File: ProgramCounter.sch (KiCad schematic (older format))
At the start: 8 parts, among them U13 74LS245, U14 74LS245, U15 74LS161, U16 74LS161, U17 74LS161, U18 74LS161

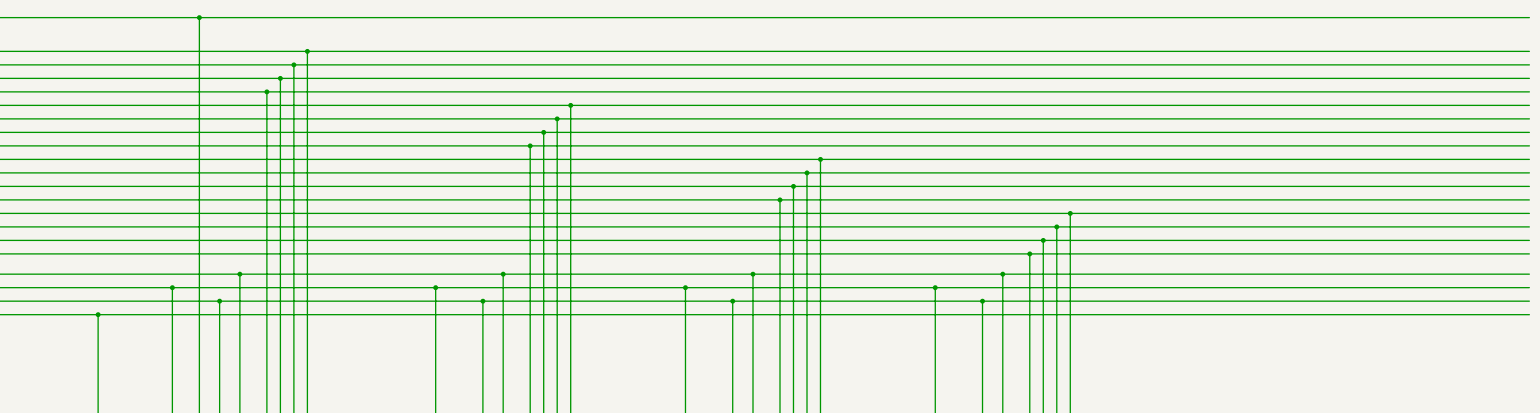
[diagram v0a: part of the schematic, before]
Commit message: clean up
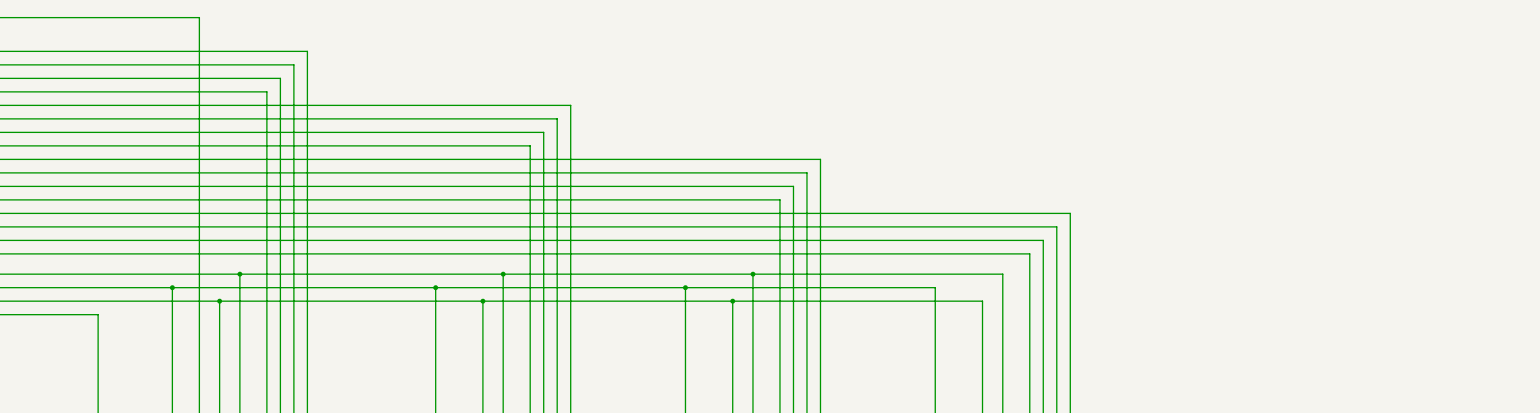
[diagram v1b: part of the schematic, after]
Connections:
- wire segments 243 -> 222
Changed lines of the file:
@@
 Wire Wire Line
 	9400 2750 11250 2750
-Connection ~ 11250 2750
-Wire Wire Line
-	11250 2750 15650 2750
 Wire Wire Line
 	1150 2750 5600 2750
@@
 Wire Wire Line
 	11750 3950 11750 2650
-Connection ~ 11750 2650
-Wire Wire Line
-	11750 2650 15650 2650
 Wire Wire Line
 	5800 3950 5800 750
-Connection ~ 5800 750
-Wire Wire Line
-	5800 750  15650 750
 Text HLabel 1150 2850 0    50   Input ~ 0
 CE
@@
 Wire Wire Line
 	11650 3900 11650 3950
-Connection ~ 11600 2850
-Wire Wire Line
-	11600 2850 15650 2850
 Wire Wire Line
 	11600 3900 11550 3900
@@
 Wire Wire Line
 	4450 5150 4450 4950
-Connection ~ 5050 2950
-Wire Wire Line
-	5050 2950 15650 2950
 Wire Wire Line
 	6600 3950 6600 1000
-Connection ~ 6600 1000
-Wire Wire Line
-	6600 1000 15650 1000
 Wire Wire Line
 	6500 3950 6500 1100
-Connection ~ 6500 1100
-Wire Wire Line
-	6500 1100 15650 1100
 Wire Wire Line
 	6400 3950 6400 1200
-Connection ~ 6400 1200
-Wire Wire Line
-	6400 1200 15650 1200
 Wire Wire Line
 	6300 3950 6300 1300
-Connection ~ 6300 1300
-Wire Wire Line
-	6300 1300 15650 1300
-Connection ~ 8550 1400
 Wire Wire Line
 	8450 1500 8450 3950
-Connection ~ 8450 1500
-Wire Wire Line
-	8450 1500 15650 1500
 Wire Wire Line
 	8350 1600 8350 3950
-Connection ~ 8350 1600
-Wire Wire Line
-	8350 1600 15650 1600
 Connection ~ 8550 3950
 Wire Wire Line
@@
 Wire Wire Line
 	2550 1700 8250 1700
-Connection ~ 8250 1700
-Wire Wire Line
-	8250 1700 15650 1700
-Wire Wire Line
-	8550 1400 15650 1400
 Wire Wire Line
 	8250 3950 8250 1700
@@
 Wire Wire Line
 	10400 3950 10400 1800
-Connection ~ 10400 1800
-Wire Wire Line
-	10400 1800 15650 1800
 Wire Wire Line
 	10300 3950 10300 1900
-Connection ~ 10300 1900
-Wire Wire Line
-	10300 1900 15650 1900
 Wire Wire Line
 	10200 3950 10200 2000
-Connection ~ 10200 2000
-Wire Wire Line
-	10200 2000 15650 2000
 Wire Wire Line
 	10100 3950 10100 2100
-Connection ~ 10100 2100
-Wire Wire Line
-	10100 2100 15650 2100
 Wire Wire Line
 	12250 3950 12250 2200
-Connection ~ 12250 2200
-Wire Wire Line
-	12250 2200 15650 2200
 Wire Wire Line
 	12150 3950 12150 2300
-Connection ~ 12150 2300
-Wire Wire Line
-	12150 2300 15650 2300
 Wire Wire Line
 	12050 3950 12050 2400
 Wire Wire Line
 	4050 2400 12050 2400
-Connection ~ 12050 2400
-Wire Wire Line
-	12050 2400 15650 2400
 Wire Wire Line
 	11950 3950 11950 2500
 Wire Wire Line
 	4150 2500 11950 2500
-Connection ~ 11950 2500
-Wire Wire Line
-	11950 2500 15650 2500
 Wire Wire Line
 	6900 4450 6900 4250
